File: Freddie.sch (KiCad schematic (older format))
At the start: 15 parts, among them J50 Test_signal, J51 To_GND, U18 74LS08, U6 Freddie, Y1 Crystal

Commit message: SMD continue
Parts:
- R20: footprint Atari:R_Axial_DIN0207_L3.6mm_D2.2mm_P10.16mm_Horizontal -> Resistor_SMD:R_1206_3216Metric_Pad1.42x1.75mm_HandSolder
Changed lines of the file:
@@
 F 0 "R20" V 8350 2700 50  0000 C CNN
 F 1 "3k" V 8275 2700 50  0000 C CNN
-F 2 "Atari:R_Axial_DIN0207_L3.6mm_D2.2mm_P10.16mm_Horizontal" V 8280 2700 50  0001 C CNN
+F 2 "Resistor_SMD:R_1206_3216Metric_Pad1.42x1.75mm_HandSolder" V 8280 2700 50  0001 C CNN
 F 3 "~" H 8350 2700 50  0001 C CNN
 	1    8350 2700

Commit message: Almost finished
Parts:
- C43: footprint Atari:C_Axial_L5.1mm_D2.5mm_P12.50mm_Horizontal -> Capacitor_SMD:C_1206_3216Metric_Pad1.42x1.75mm_HandSolder
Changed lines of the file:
@@
 F 0 "C43" H 10925 2800 50  0000 L CNN
 F 1 "100nF" H 10925 2600 50  0000 L CNN
-F 2 "Atari:C_Axial_L5.1mm_D2.5mm_P12.50mm_Horizontal" H 10938 2550 50  0001 C CNN
+F 2 "Capacitor_SMD:C_1206_3216Metric_Pad1.42x1.75mm_HandSolder" H 10938 2550 50  0001 C CNN
 F 3 "~" H 10900 2700 50  0001 C CNN
 	1    10900 2700

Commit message: gerber
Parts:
- R30: footprint Atari:R_Axial_DIN0207_L3.6mm_D2.2mm_P10.16mm_Horizontal -> Resistor_SMD:R_1206_3216Metric_Pad1.42x1.75mm_HandSolder
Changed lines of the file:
@@
 F 0 "R30" H 5630 1729 50  0000 R CNN
 F 1 "3k" H 5630 1820 50  0000 R CNN
-F 2 "Atari:R_Axial_DIN0207_L3.6mm_D2.2mm_P10.16mm_Horizontal" V 5630 1775 50  0001 C CNN
+F 2 "Resistor_SMD:R_1206_3216Metric_Pad1.42x1.75mm_HandSolder" V 5630 1775 50  0001 C CNN
 F 3 "~" H 5700 1775 50  0001 C CNN
 	1    5700 1775

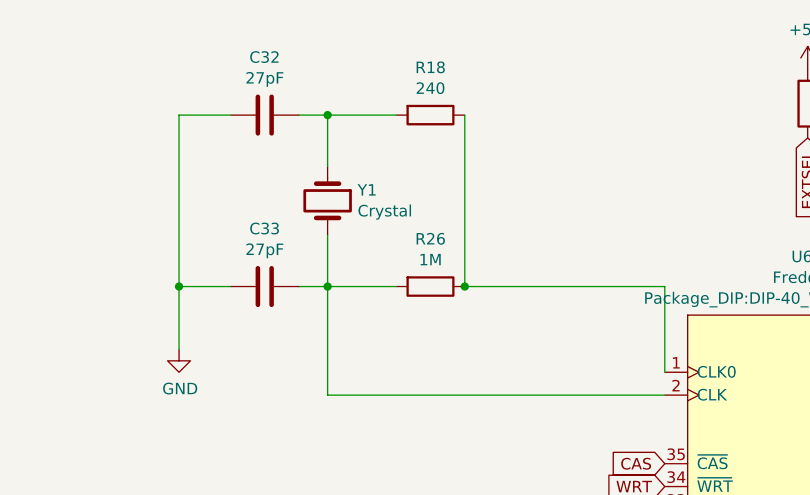
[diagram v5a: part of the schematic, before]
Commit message: Final inspection
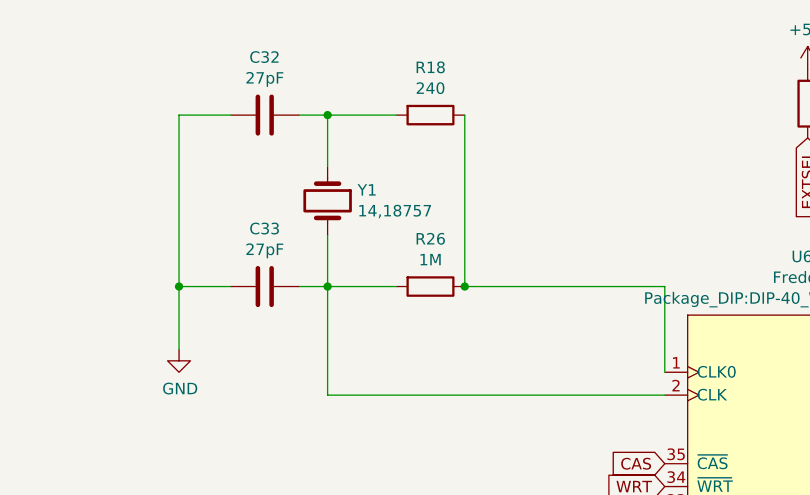
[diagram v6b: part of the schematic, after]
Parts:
- Y1: value Crystal -> 14,18757
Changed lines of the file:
@@
 P 3600 2200
 F 0 "Y1" V 3554 2331 50  0000 L CNN
-F 1 "Crystal" V 3645 2331 50  0000 L CNN
+F 1 "14,18757" V 3645 2331 50  0000 L CNN
 F 2 "Crystal:Crystal_HC18-U_Vertical" H 3600 2200 50  0001 C CNN
 F 3 "~" H 3600 2200 50  0001 C CNN
